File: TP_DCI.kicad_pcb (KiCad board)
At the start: 2 copper layers, 35 parts, among them SW1 SW_DIP_x03, U1 MAX3157CAI+, U2 TPS54232, X1 Screw_Terminal_01x06, X2 Screw_Terminal_01x02

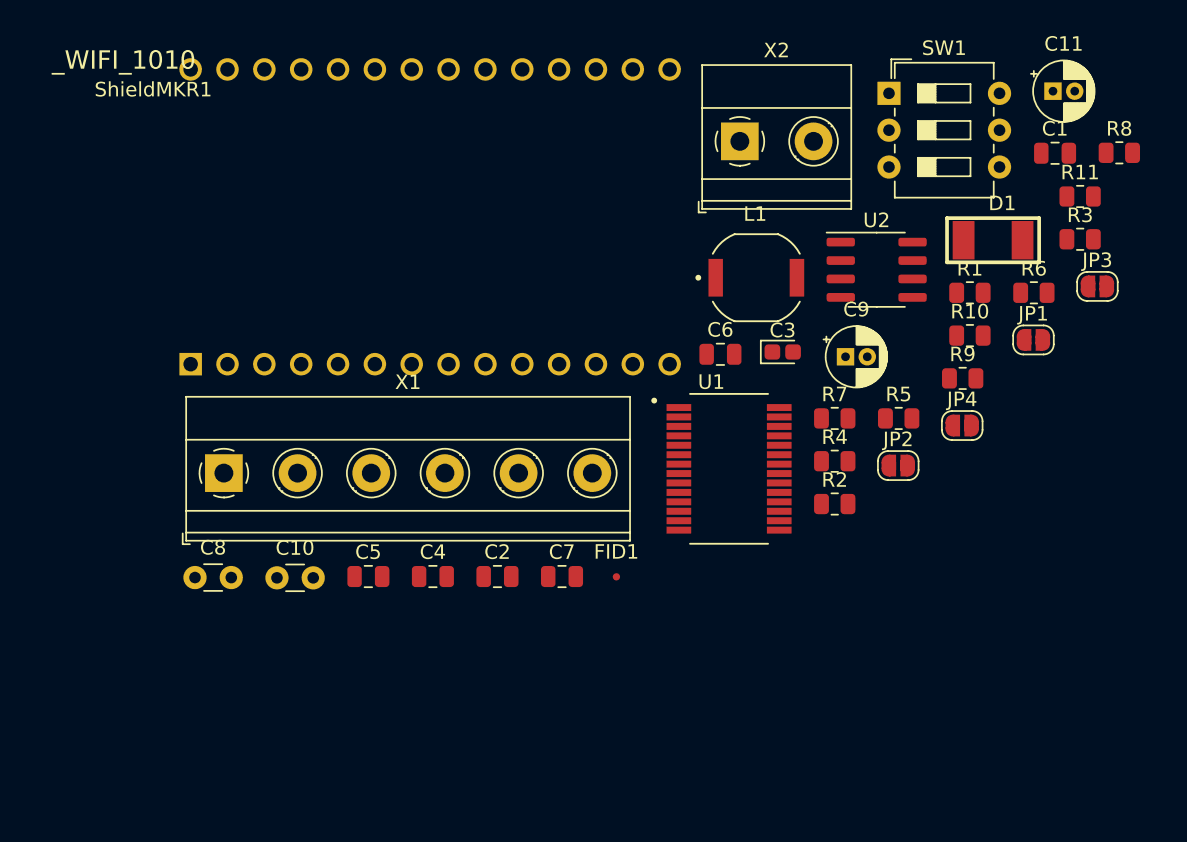
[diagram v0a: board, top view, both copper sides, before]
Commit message: Para correccion Etapa 1
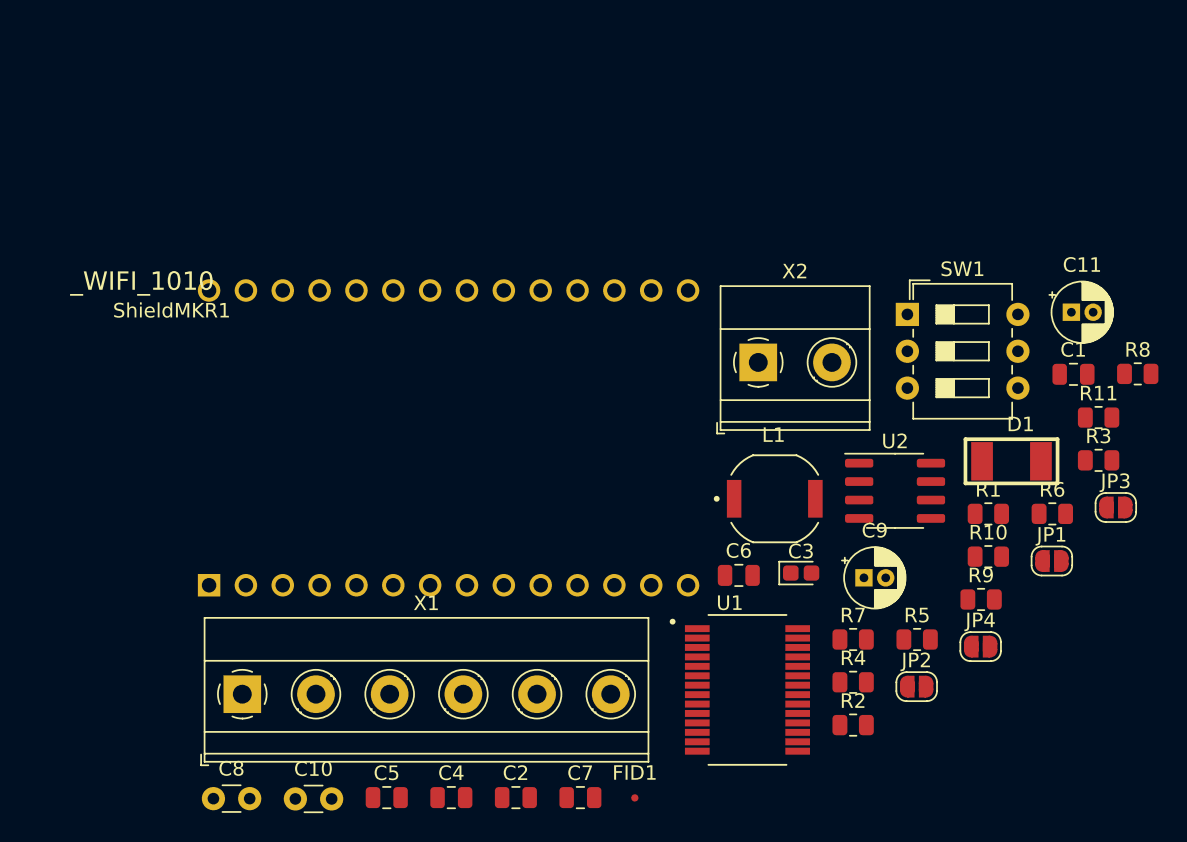
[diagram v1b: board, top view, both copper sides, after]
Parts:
- moved C3 15.3 mm to (152.7, 100.1)
- moved C7 15.3 mm to (137.5, 115.5)
- moved FID1 15.3 mm to (141.2, 115.6)
- moved JP1 15.3 mm to (170.0, 99.2)
- moved JP3 15.3 mm to (174.4, 95.5)
- moved R1 15.3 mm to (165.6, 96.0)
- moved R10 15.3 mm to (165.6, 98.9)
- moved R11 15.3 mm to (173.2, 89.3)
- moved R3 15.3 mm to (173.2, 92.3)
- moved R6 15.3 mm to (170.0, 96.0)
- moved SW1 15.3 mm to (160.0, 82.2)
- moved X2 15.3 mm to (149.7, 85.5)
- moved C2 15.3 mm to (133.0, 115.5)
- moved C4 15.3 mm to (128.6, 115.5)
- moved C5 15.3 mm to (124.1, 115.5)
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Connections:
- C2 pad 2: Net-(C2-Pad2) -> /ISOGND
- R11 pad 1: Net-(R11-Pad1) -> /H_#F
- R11 pad 2: /Y -> /ISOVCC
- R2 pad 1: GND -> /Y
- R2 pad 2: /H_#F -> Net-(R2-Pad2)
- SW1 pad 2: Net-(R11-Pad1) -> /H_#F
- SW1 pad 3: /H_#F -> Net-(R2-Pad2)
- U1 pad 14: Net-(C2-Pad2) -> /ISOGND
